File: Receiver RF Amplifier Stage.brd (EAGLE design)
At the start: 115.5 x 84.8 mm, 15 parts, among them T1 2N2222

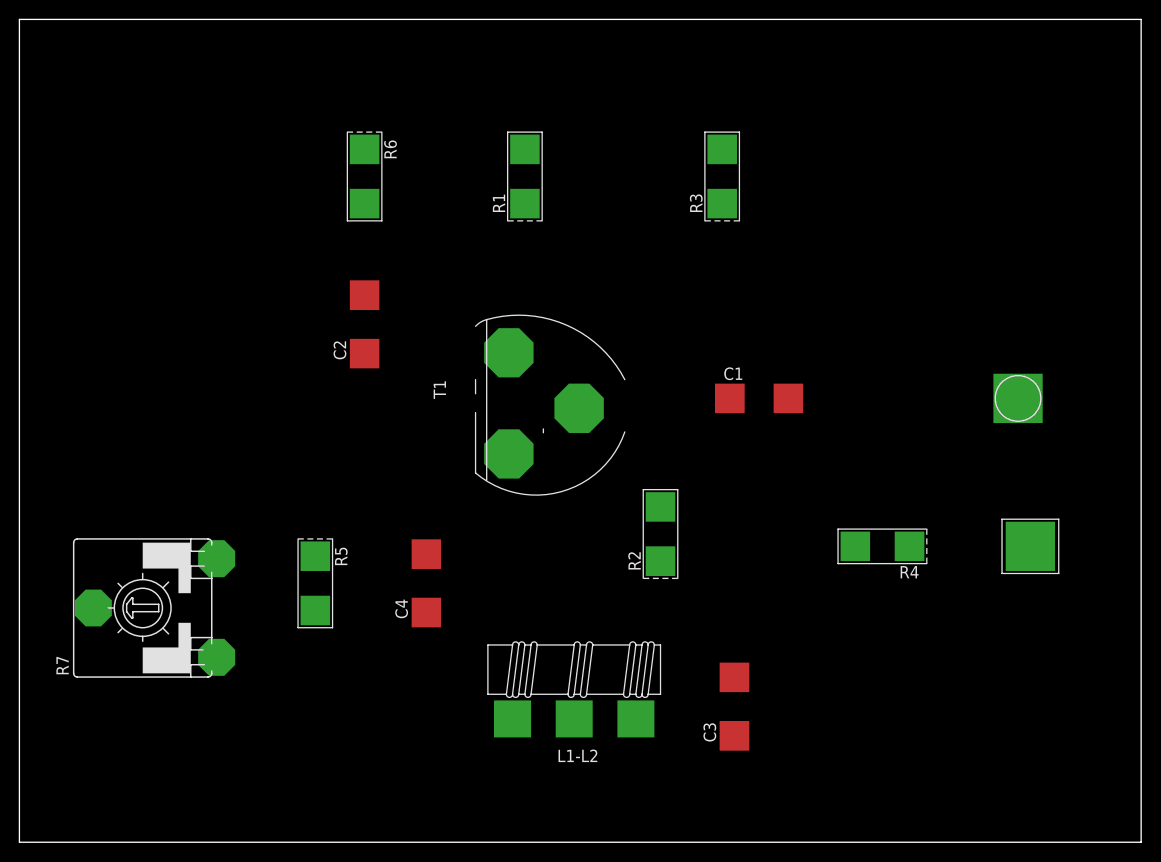
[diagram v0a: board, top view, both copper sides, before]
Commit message: Lots of changes.
Recreated the IF Schema and a new board to look like the photo

On branch master
Changes to be committed:
       modified:   Receiver RF Amplifier Stage.b#1
       modified:   Receiver RF Amplifier Stage.b#2
       modified:   Receiver RF Amplifier Stage.b#3
       modified:   Receiver RF Amplifier Stage.b#4
       modified:   Receiver RF Amplifier Stage.b#5
       modified:   Receiver RF Amplifier Stage.b#6
       modified:   Receiver RF Amplifier Stage.b#7
       modified:   Receiver RF Amplifier Stage.b#8
       modified:   Receiver RF Amplifier Stage.b#9
       modified:   Receiver RF Amplifier Stage.brd
       modified:   Receiver RF Amplifier Stage.s#1
       modified:   Receiver RF Amplifier Stage.s#2
       modified:   Receiver RF Amplifier Stage.s#3
       modified:   Receiver RF Amplifier Stage.s#4
       modified:   Receiver RF Amplifier Stage.s#5
       modified:   Receiver RF Amplifier Stage.s#6
       modified:   Receiver RF Amplifier Stage.s#7
       modified:   Receiver RF Amplifier Stage.s#8
       modified:   Receiver RF Amplifier Stage.s#9
       modified:   Receiver RF Amplifier Stage.sch
       modified:   Sudden_XCVR_IF_Module.b#1
       modified:   Sudden_XCVR_IF_Module.b#2
       modified:   Sudden_XCVR_IF_Module.b#3
       modified:   Sudden_XCVR_IF_Module.b#4
       modified:   Sudden_XCVR_IF_Module.b#5
       modified:   Sudden_XCVR_IF_Module.b#6
       modified:   Sudden_XCVR_IF_Module.b#7
       modified:   Sudden_XCVR_IF_Module.brd
       new file:   Sudden_XCVR_IF_Module_Schematic_like_board_layout.b#1
       new file:   Sudden_XCVR_IF_Module_Schematic_like_board_layout.b#2
       new file:   Sudden_XCVR_IF_Module_Schematic_like_board_layout.b#3
       new file:   Sudden_XCVR_IF_Module_Schematic_like_board_layout.brd
       new file:   Sudden_XCVR_IF_Module_Schematic_like_board_layout.s#1
       new file:   Sudden_XCVR_IF_Module_Schematic_like_board_layout.s#2
       new file:   Sudden_XCVR_IF_Module_Schematic_like_boa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
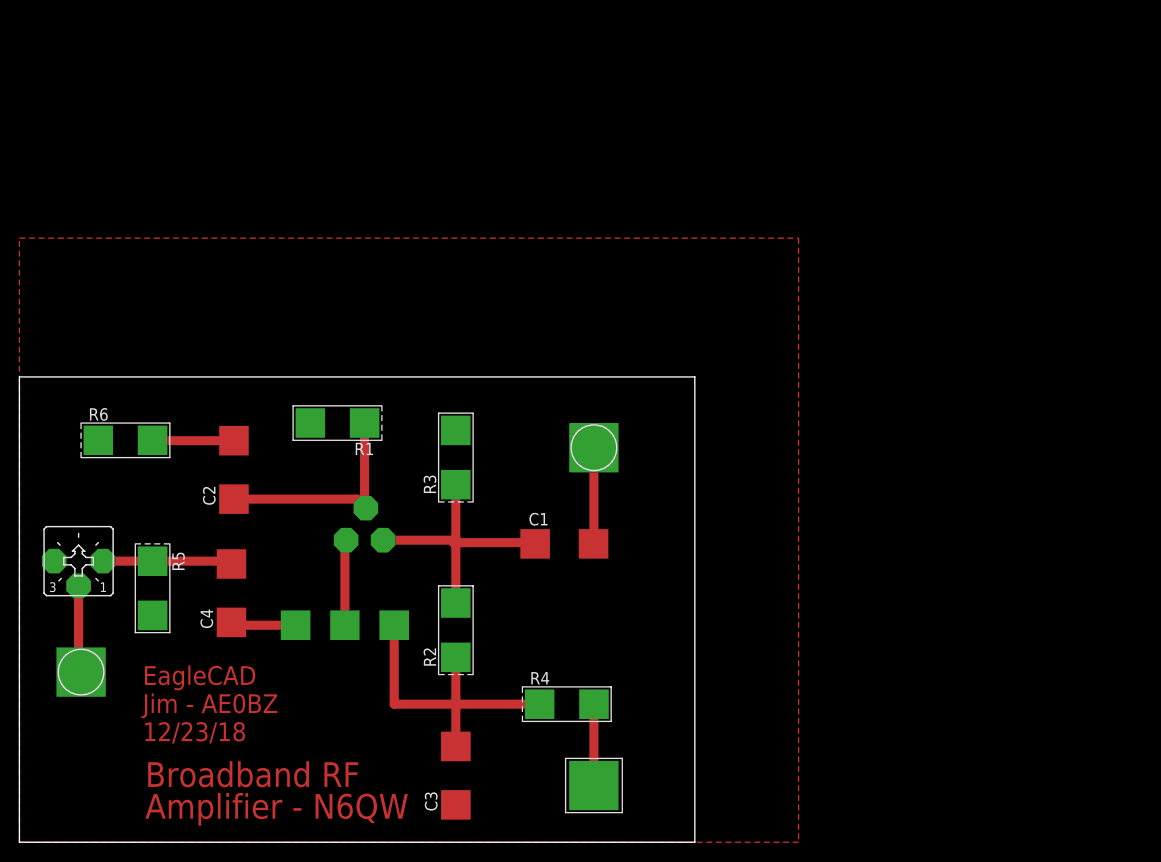
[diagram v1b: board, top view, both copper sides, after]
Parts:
- removed R7: 100R, jim_muppet_parts:CA14V
- added AC-SIGNAL-OUT: Output from Center Wiper, jim_muppet_parts:PAD-SQUARE
- added R11: (no value), jim_muppet_parts:POT-TRIMM-4
- T1: device jim_muppet_parts:TO92 -> jim_muppet_parts:2N2222-TO18
- moved P+1 51.3 mm to (59.2, 5.84)
- moved AC-SIGNAL 44.0 mm to (59.2, 40.6)
- moved R3 39.9 mm to (45.0, 39.6)
- moved R6 36.7 mm to (10.9, 41.4), turned to 0 degrees
- moved R4 36.3 mm to (56.4, 14.2), turned to 0 degrees
- moved R1 31.9 mm to (32.8, 43.2), turned to 180 degrees
- moved C3 29.6 mm to (45.0, 6.86)
- moved C1 25.0 mm to (56.1, 30.7)
- moved L1-L2 23.6 mm to (33.5, 17.3), flipped to the bottom, turned to 270 degrees
- moved R2 23.3 mm to (45.0, 21.8)
- moved T1 22.1 mm to (35.6, 34.5), flipped to the bottom
- moved C2 20.1 mm to (22.1, 38.4)
- moved C4 20.1 mm to (21.8, 25.7)
- moved R5 16.8 mm to (13.7, 26.2)
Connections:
- new net N$3: AC-SIGNAL-OUT.PAD, R11.S
- net GND: now also R11.E; no longer R7.A
- net N$8: now also R11.A; no longer R7.E
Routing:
- net N$7: track 0.00 -> 33.0 mm
- net N$1: track 0.00 -> 28.8 mm
- net N$12: track 0.00 -> 23.1 mm
- net N$8: track 0.00 -> 15.1 mm
- net N$9: track 0.00 -> 9.92 mm
- net N$3: track 0.00 -> 9.14 mm
- net N$5: track 0.00 -> 8.89 mm
- net N$4: track 0.00 -> 8.67 mm
- net +12V: track 0.00 -> 8.38 mm
- net N$6: track 0.00 -> 6.73 mm
- added copper zone on layer 1, net GND
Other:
- board size 115.5 x 84.8 mm -> 69.6 x 47.9 mm
- board text added: "Broadband RF Amplifier - N6QW"
- board text added: "EagleCAD Jim - AE0BZ 12/23/18"
